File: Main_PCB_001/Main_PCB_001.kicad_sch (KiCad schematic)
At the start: 69 parts, among them IC1 FDN8601, IC2 FDN8601, IC3 TPS40211QDGQRQ1, IC4 PAM2863ECR, IC5 FDN8601, IC6 ZXTR2105FQ-7, U1 ATtiny25-20S, U2 Mounting_Hole_M2, U3 Mounting_Hole_M2, U4 Mounting_Hole_M2, U5 Mounting_Hole_M2

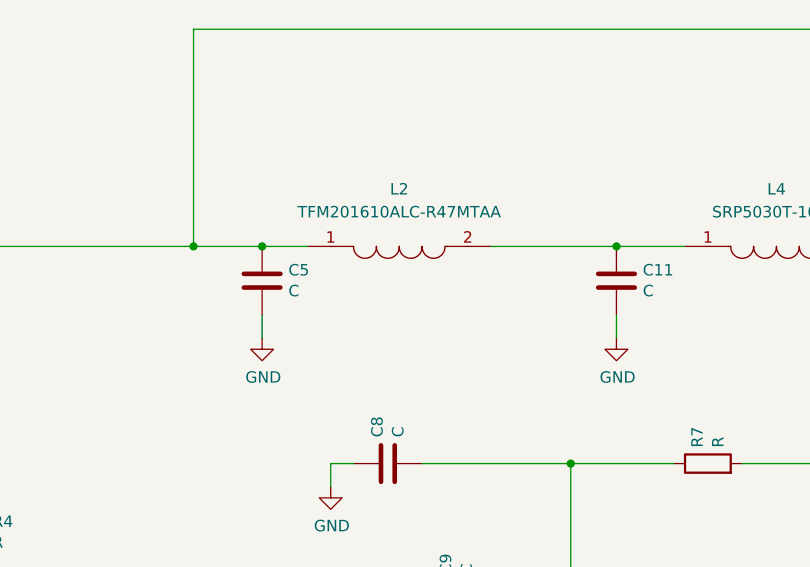
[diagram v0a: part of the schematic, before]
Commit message: PCB underwork
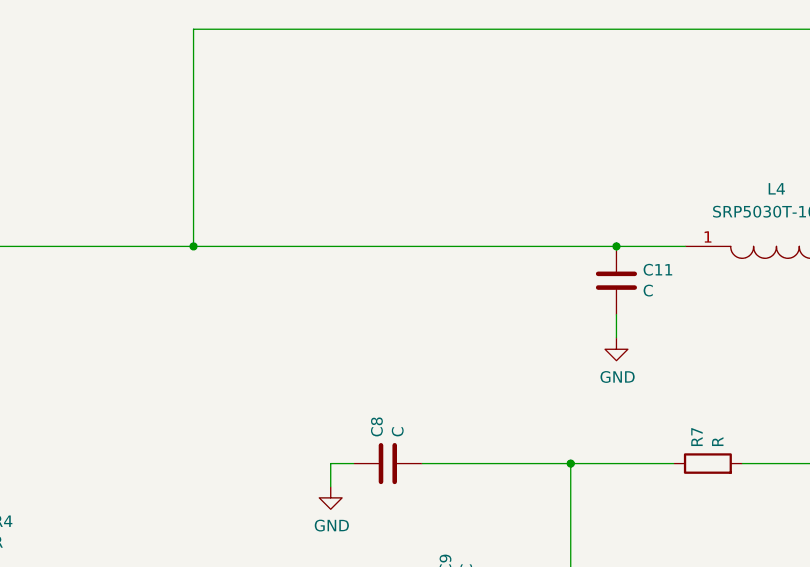
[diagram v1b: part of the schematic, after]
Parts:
- removed C5: C, Capacitor_SMD:C_0603_1608Metric, symbol Device:C
- removed L2: TFM201610ALC-R47MTAA, libraries:INDC2016X80N, symbol TFM201610ALC-R47MTAA:TFM201610ALC-R47MTAA
- C15, C4, C6, C8, C9: footprint Capacitor_SMD:C_0603_1608Metric_Pad1.08x0.95mm_HandSolder -> (none)
- C20: footprint (none) -> Capacitor_SMD:C_1206_3216Metric_Pad1.33x1.80mm_HandSolder
- L4: footprint libraries:INDPM5752X300N -> (none)
- L7: footprint libraries:INDPM7366X500N -> (none)
- R10, R11, R4, R5, R7, R8, R9: footprint Resistor_SMD:R_0603_1608Metric_Pad0.98x0.95mm_HandSolder -> (none)
- R3: footprint Resistor_SMD:R_1206_3216Metric_Pad1.30x1.75mm_HandSolder -> (none)
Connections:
- net at C21.1, D1.1 (Conn), L10.1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: now also C11.1, L4.1

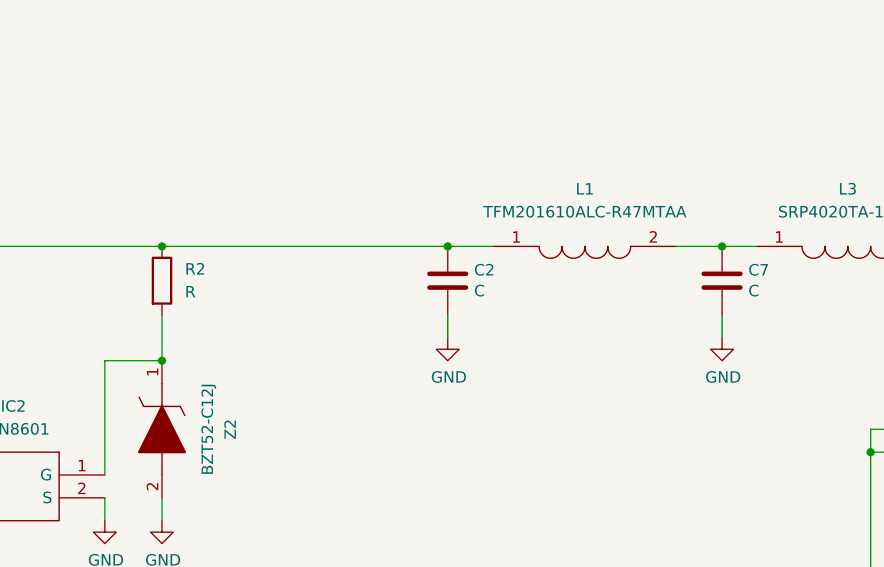
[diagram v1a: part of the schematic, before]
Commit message: PCB working on
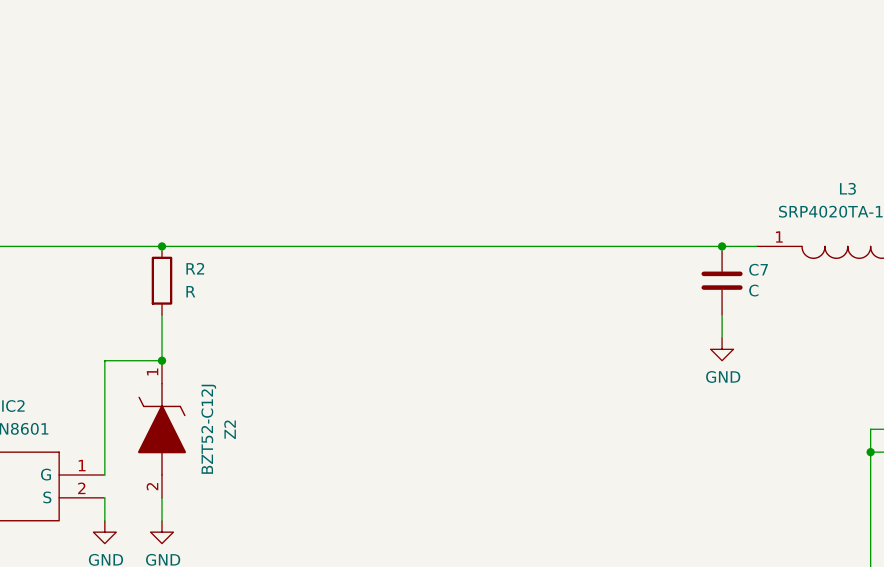
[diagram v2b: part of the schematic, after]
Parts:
- removed C2: C, Capacitor_SMD:C_0603_1608Metric_Pad1.08x0.95mm_HandSolder, symbol Device:C
- removed L1: TFM201610ALC-R47MTAA, libraries:INDC2016X80N, symbol TFM201610ALC-R47MTAA:TFM201610ALC-R47MTAA
- C10, C20: footprint Capacitor_SMD:C_1206_3216Metric_Pad1.33x1.80mm_HandSolder -> (none)
- C15, C4, C6, C8, C9: footprint (none) -> Capacitor_SMD:C_0402_1005Metric_Pad0.74x0.62mm_HandSolder
- L3: footprint libraries:INDPM4441X200N -> (none)
- L4: footprint (none) -> libraries:INDPM4441X200N
- L7: footprint (none) -> libraries:INDPM5752X300N
- R10: footprint (none) -> Resistor_SMD:R_0603_1608Metric_Pad0.98x0.95mm_HandSolder
- R3: footprint (none) -> Resistor_SMD:R_0805_2012Metric_Pad1.20x1.40mm_HandSolder
- R4, R5, R7, R8, R9: footprint (none) -> Resistor_SMD:R_0402_1005Metric_Pad0.72x0.64mm_HandSolder
- U2, U3, U4, U5: footprint mount_holes:Hole_screw_M2 -> (none)
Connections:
- net at D2.1 (Conn), R2.1: now also C7.1, L3.1

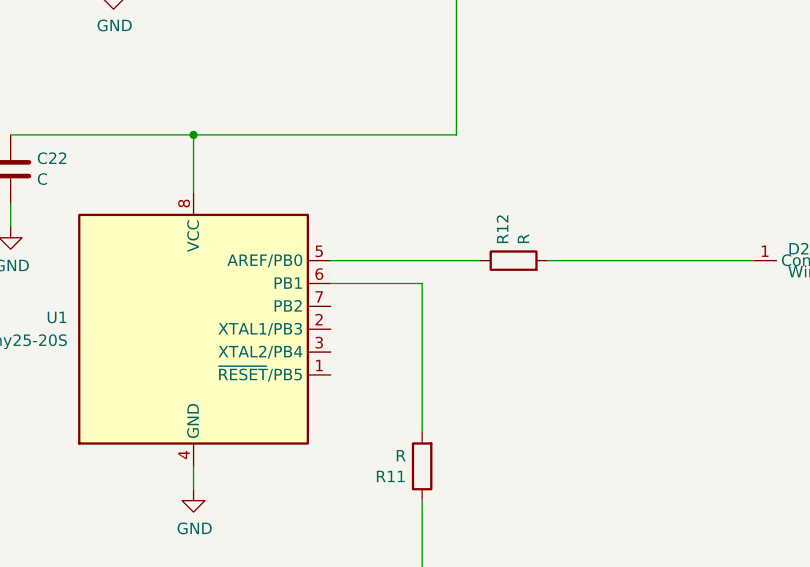
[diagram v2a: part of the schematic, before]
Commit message: PCB working on
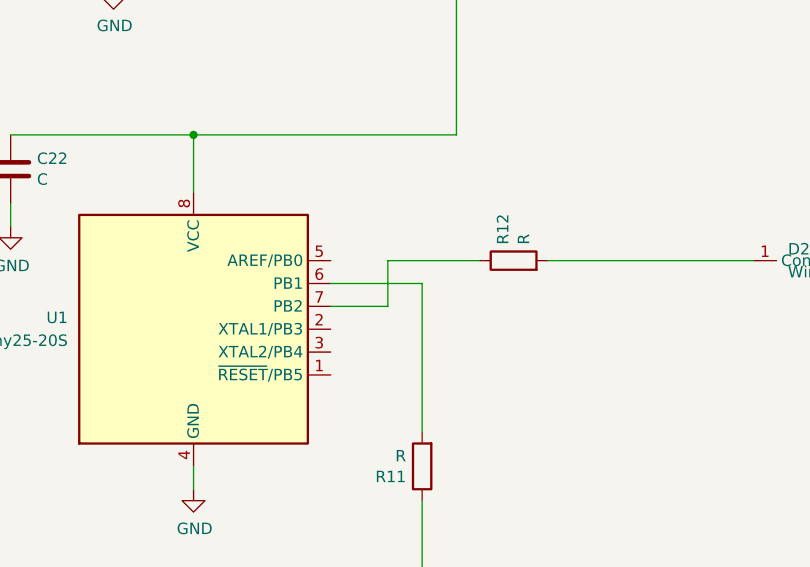
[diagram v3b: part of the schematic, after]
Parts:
- C10, C20: footprint (none) -> Capacitor_SMD:C_0805_2012Metric_Pad1.18x1.45mm_HandSolder
- L3: footprint (none) -> libraries:INDC2016X80N
- R11: footprint (none) -> Resistor_SMD:R_0603_1608Metric_Pad0.98x0.95mm_HandSolder
- U2, U3, U4, U5: footprint (none) -> mount_holes:Hole_screw_M1p2
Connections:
- net at R12.1: now also U1.7 (PB2); no longer U1.5 (AREF/PB0)
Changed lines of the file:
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@@
+    (stroke (width 0) (type default) (color 0 0 0 0))
+  )
+  (wire (pts (xy 412.75 105.41) (xy 412.75 100.33))
     (stroke (width 0) (type default) (color 0 0 0 0))
   )
@@
     (stroke (width 0) (type default) (color 0 0 0 0))
   )
+  (wire (pts (xy 412.75 100.33) (xy 422.91 100.33))
+    (stroke (width 0) (type default) (color 0 0 0 0))
+  )
+  (wire (pts (xy 406.4 105.41) (xy 412.75 105.41))
+    (stroke (width 0) (type default) (color 0 0 0 0))
+  )
   (wire (pts (xy 173.99 250.19) (xy 186.69 250.19))
     (stroke (width 0) (type default) (color 0 0 0 0))
@@
   )
   (wire (pts (xy 222.25 250.19) (xy 233.68 250.19))
-    (stroke (width 0) (type default) (color 0 0 0 0))
-  )
-  (wire (pts (xy 406.4 100.33) (xy 422.91 100.33))
     (stroke (width 0) (type default) (color 0 0 0 0))
   )
@@
       (effects (font (size 1.27 1.27)) (justify left))
     )
-    (property "Footprint" "" (id 2) (at 414.02 259.08 0)
+    (property "Footprint" "mount_holes:Hole_screw_M1p2" (id 2) (at 414.02 259.08 0)
       (effects (font (size 1.27 1.27)) hide)
     )
@@
     (property "Reference" "L3" (id 0) (at 161.29 223.52 0))
     (property "Value" "SRP4020TA-100M" (id 1) (at 161.29 226.06 0))
-    (property "Footprint" "" (id 2) (at 167.64 228.6 0)
+    (property "Footprint" "libraries:INDC2016X80N" (id 2) (at 167.64 228.6 0)
       (effects (font (size 1.27 1.27)) (justify left) hide)
     )
@@
       (effects (font (size 1.27 1.27)) (justify left))
     )
-    (property "Footprint" "" (id 2) (at 414.02 274.32 0)
+    (property "Footprint" "mount_holes:Hole_screw_M1p2" (id 2) (at 414.02 274.32 0)
       (effects (font (size 1.27 1.27)) hide)
     )
@@
       (effects (font (size 1.27 1.27)) (justify left))
     )
-    (property "Footprint" "" (id 2) (at 284.1752 265.43 0)
+    (property "Footprint" "Capacitor_SMD:C_0805_2012Metric_Pad1.18x1.45mm_HandSolder" (id 2) (at 284.1752 265.43 0)
       (effects (font (size 1.27 1.27)) hide)
     )
@@
       (effects (font (size 1.27 1.27)) (justify left))
     )
-    (property "Footprint" "" (id 2) (at 414.02 251.46 0)
+    (property "Footprint" "mount_holes:Hole_screw_M1p2" (id 2) (at 414.02 251.46 0)
       (effects (font (size 1.27 1.27)) hide)
     )
@@
       (effects (font (size 1.27 1.27)) (justify left))
     )
-    (property "Footprint" "" (id 2) (at 418.338 123.19 90)
+    (property "Footprint" "Resistor_SMD:R_0603_1608Metric_Pad0.98x0.95mm_HandSolder" (id 2) (at 418.338 123.19 90)
       (effects (font (size 1.27 1.27)) hide)
     )
@@
       (effects (font (size 1.27 1.27)) (justify left))
     )
-    (property "Footprint" "" (id 2) (at 414.02 266.7 0)
+    (property "Footprint" "mount_holes:Hole_screw_M1p2" (id 2) (at 414.02 266.7 0)
       (effects (font (size 1.27 1.27)) hide)
     )
@@
       (effects (font (size 1.27 1.27)) (justify left))
     )
-    (property "Footprint" "" (id 2) (at 177.4952 237.49 0)
-      (effects (font (size 1.27 1.27)) hide)
-    )
+    (property "Footprint" "Capacitor_SMD:C_0805_2012Metric_Pad1.18x1.45mm_HandSolder" (id 2) (at 177.4952 237.49 0)
+      (effects (font (size 1.27 1.27)) hide)
+    )
